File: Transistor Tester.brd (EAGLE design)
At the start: 160 x 100 mm, 23 parts, among them Q1 BC547

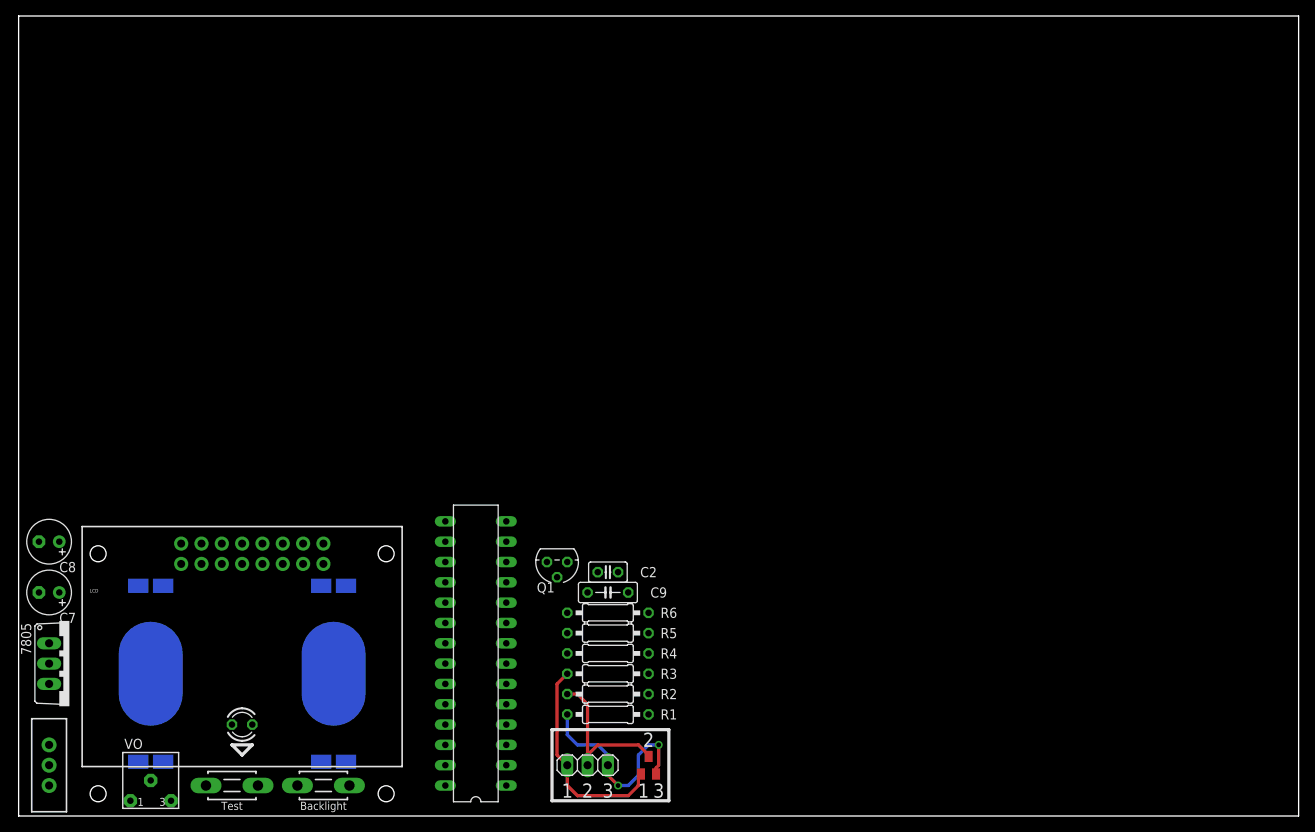
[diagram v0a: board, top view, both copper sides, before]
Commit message: Time to start routing
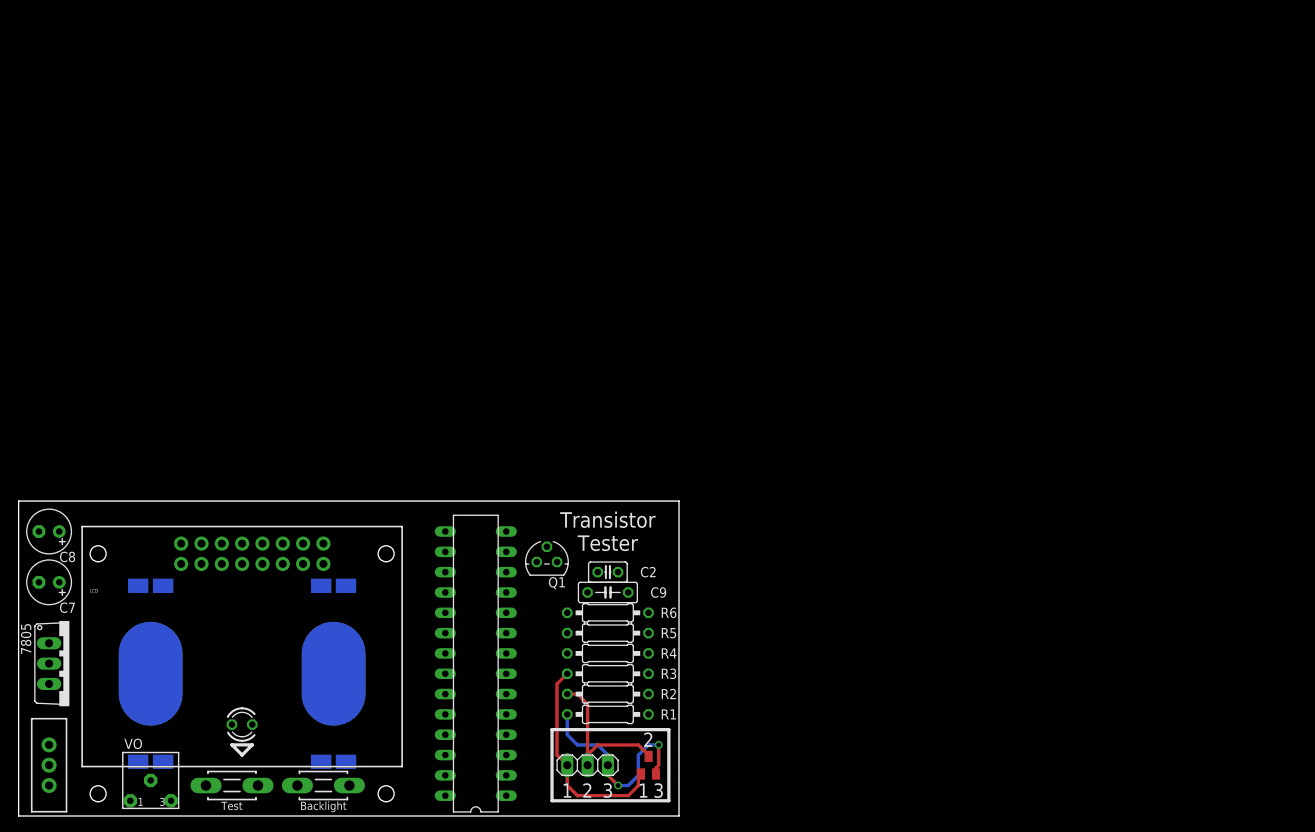
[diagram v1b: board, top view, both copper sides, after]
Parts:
- moved C8 1.27 mm to (3.81, 35.6)
- moved C7 1.27 mm to (3.81, 29.2)
- moved MCU 1.27 mm to (57.1, 19.1)
- moved Q1 1.27 mm to (66.0, 31.8), turned to 0 degrees
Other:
- board size 160 x 100 mm -> 82.5 x 39.4 mm
- board text added: "Nathan Campos, 2013"
- board text added: "Transistor Tester"
